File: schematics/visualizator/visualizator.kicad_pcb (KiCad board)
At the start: 2 copper layers, 41.9 x 43.2 mm, 20 parts, among them J1 5V, J2 WS2812, J3 Audio, SW1 COLOR, SW2 PATTERN, U1 ATmega328-16PU, Y1 16MHz

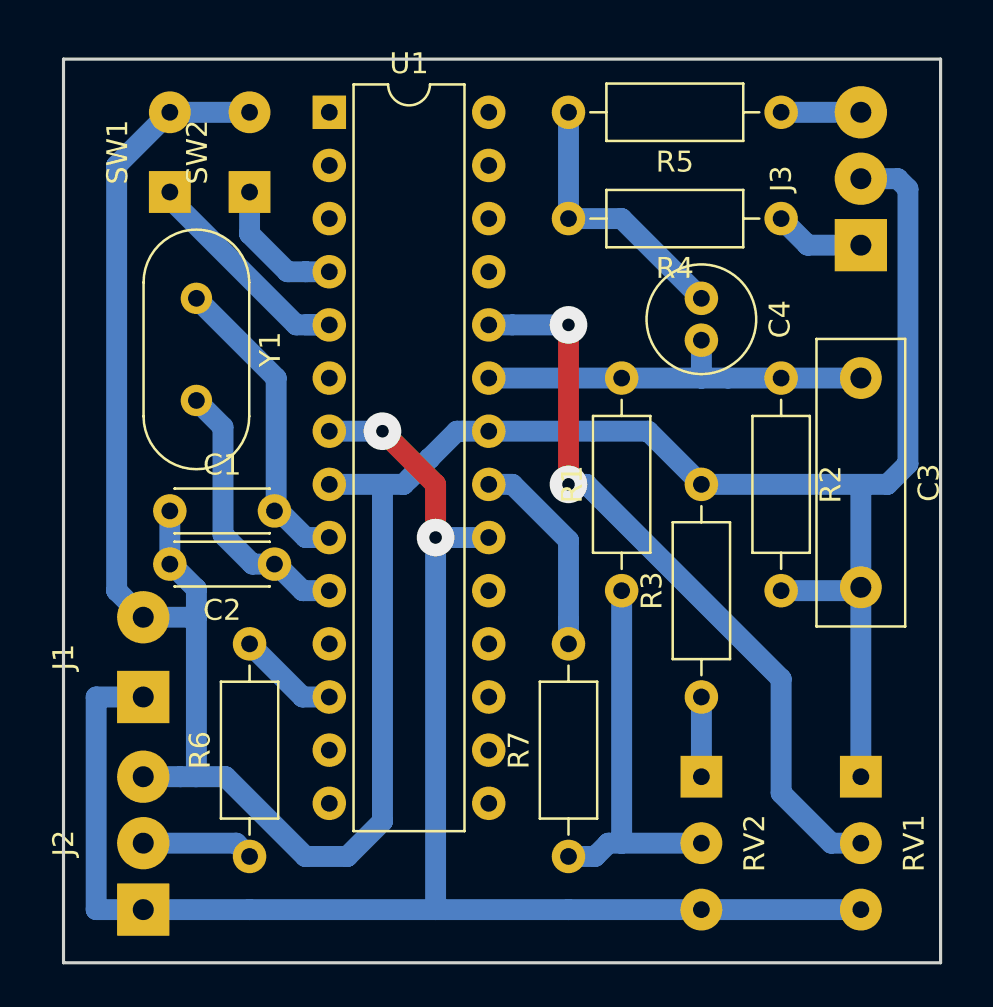
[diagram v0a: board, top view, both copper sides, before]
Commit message: PCB updated
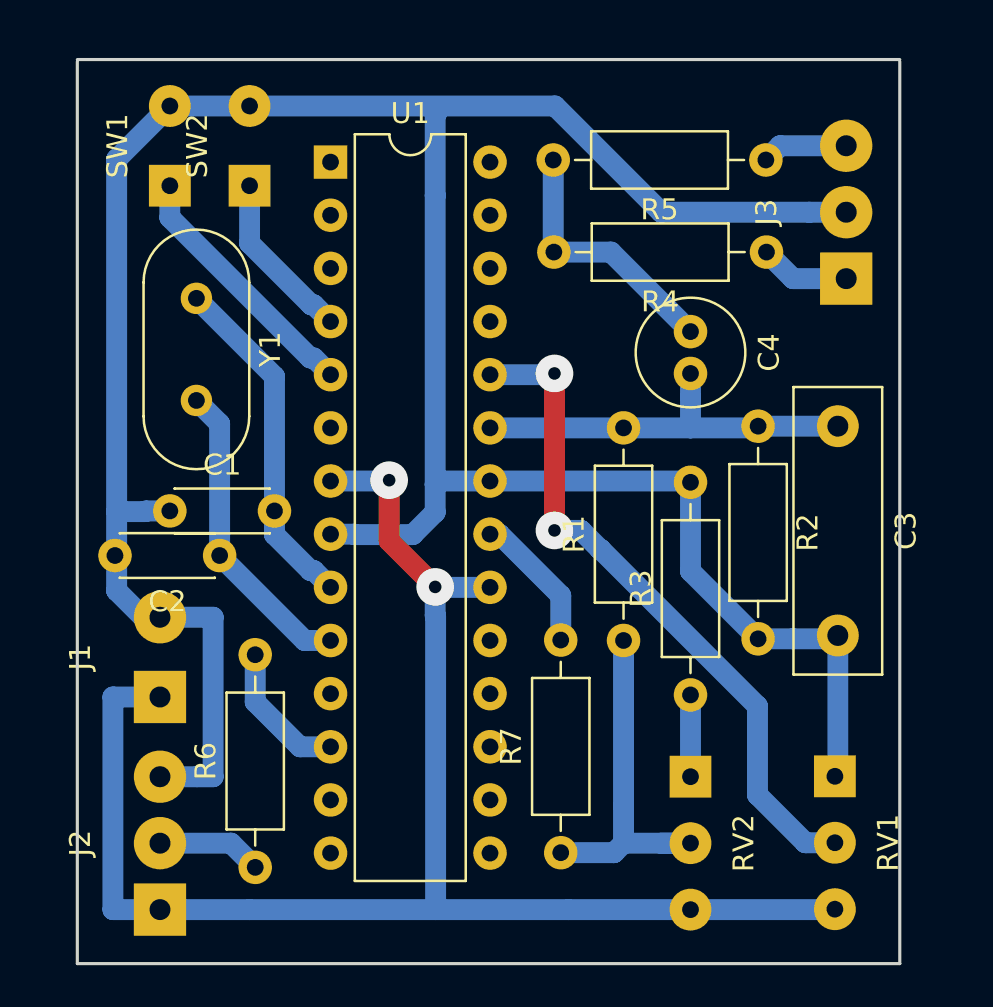
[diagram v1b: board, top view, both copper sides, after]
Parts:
- moved C2 2.65 mm to (60.8, 54.2)
- moved C3 2.55 mm to (90.3, 48.0)
- moved R2 2.55 mm to (86.5, 48.0)
- moved R5 2.39 mm to (86.9, 35.3)
- moved R1 2.38 mm to (80.1, 58.3)
- moved U1 2.38 mm to (66.1, 35.4)
- moved J3 1.75 mm to (90.7, 41.0)
- moved R4 1.75 mm to (86.9, 39.7)
- moved C4 1.67 mm to (83.3, 43.5)
- moved RV1 1.24 mm to (90.2, 64.8)
- moved J1 0.80 mm to (58.0, 61.0)
- moved J2 0.80 mm to (58.0, 71.1)
- moved R6 0.59 mm to (62.5, 69.1)
- moved R3 0.53 mm to (83.3, 60.9)
- moved RV2 0.52 mm to (83.3, 64.8)
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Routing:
- net Net-(C1-Pad1): track 140.0 -> 132.1 mm
- net Net-(J1-Pad1): track 77.9 -> 74.6 mm
- net Net-(R7-Pad2): track 9.86 -> 6.72 mm
- net Net-(RV1-Pad2): track 35.7 -> 32.7 mm
- net Net-(R6-Pad2): track 4.86 -> 6.75 mm
- net Net-(C1-Pad2): track 14.7 -> 16.6 mm
- net Net-(C2-Pad1): track 13.1 -> 14.9 mm
- net Net-(SW2-Pad1): track 6.56 -> 7.87 mm
- net Net-(R1-Pad1): track 18.7 -> 17.5 mm
- net Net-(SW1-Pad1): track 11.6 -> 12.3 mm
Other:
- board size 41.9 x 43.2 mm -> 39.3 x 43.2 mm
